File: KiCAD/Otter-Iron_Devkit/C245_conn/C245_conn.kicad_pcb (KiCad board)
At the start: 2 copper layers, 24.7 x 20.4 mm, 3 parts, among them J1 Otter-Iron, J2 C245

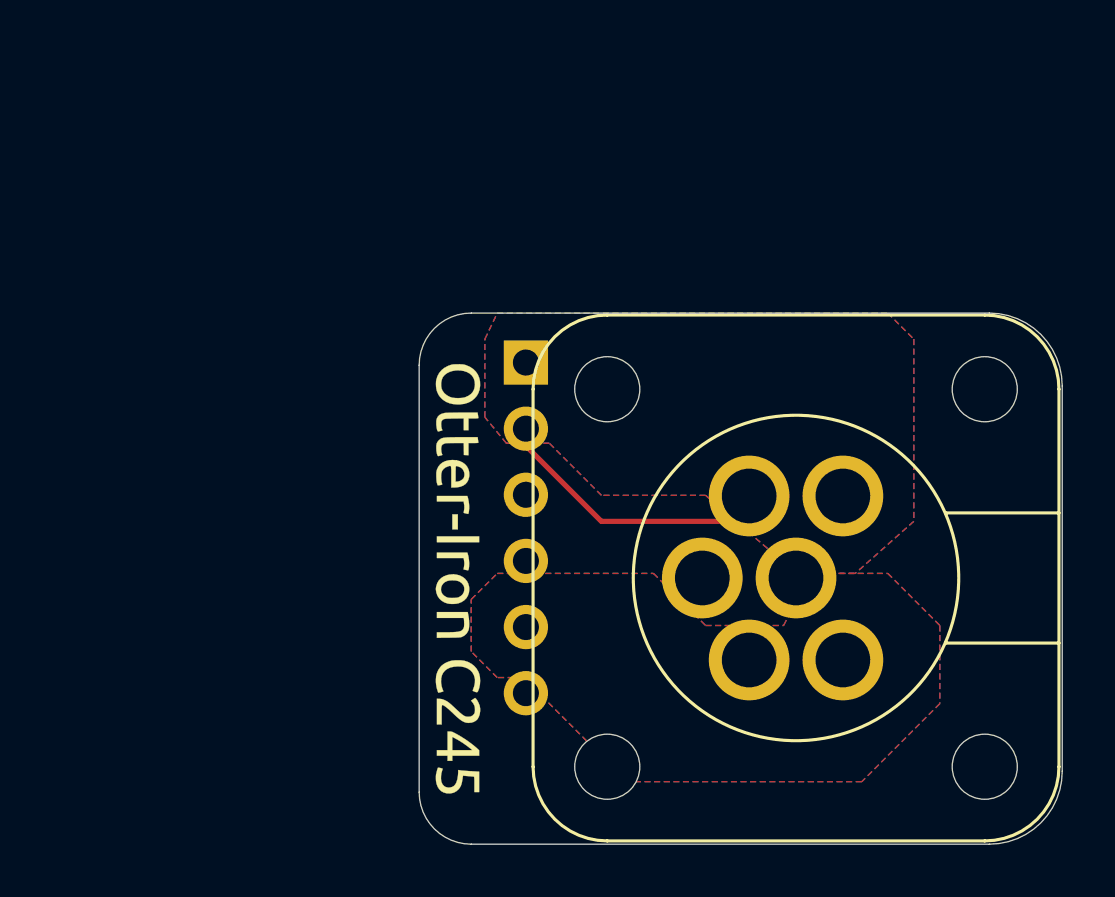
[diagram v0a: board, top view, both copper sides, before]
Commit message: added v2.0
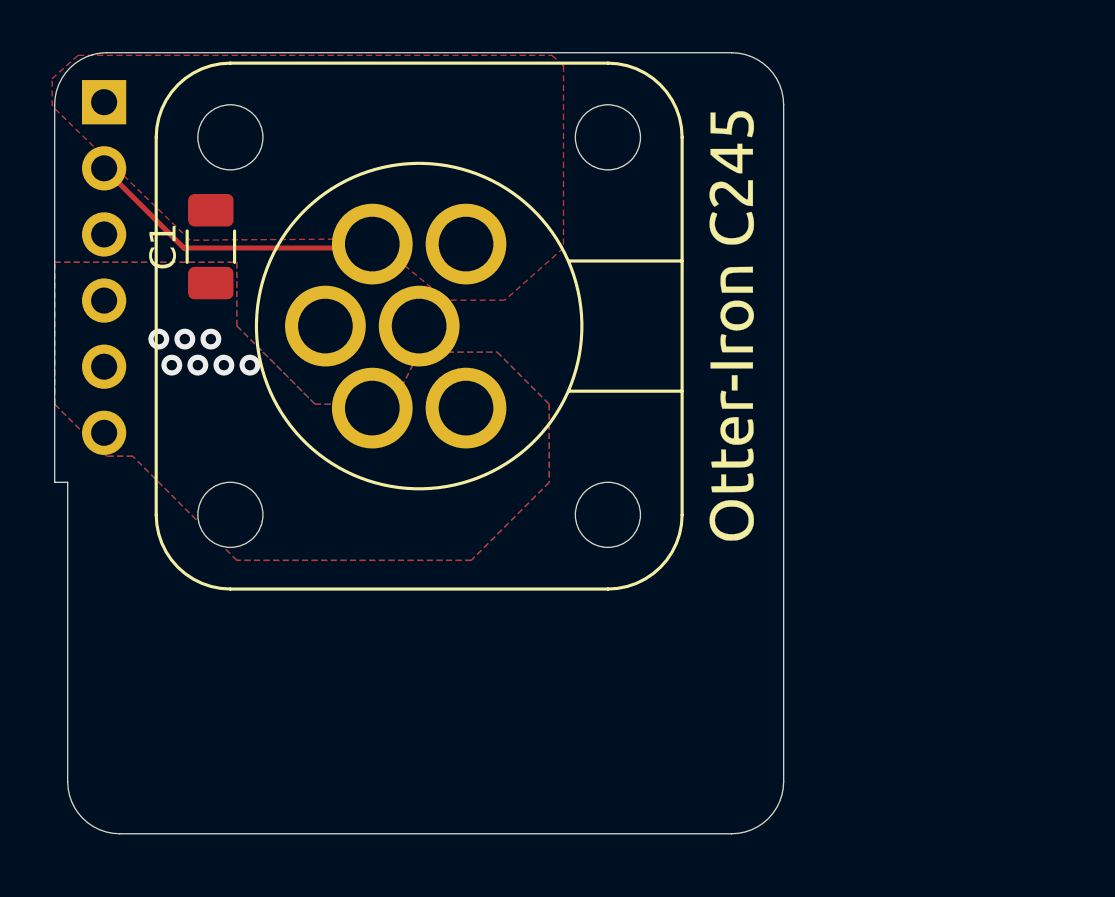
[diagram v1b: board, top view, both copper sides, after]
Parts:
- added C1: 10u, Capacitor_SMD:C_1206_3216Metric, F.Cu at (92.0, 97.5)
- J1: footprint Connector_PinHeader_2.54mm:PinHeader_1x06_P2.54mm_Horizontal -> Connector_PinHeader_2.54mm:PinHeader_1x06_P2.54mm_Vertical
- moved J1 19.0 mm to (87.9, 91.9)
- moved J2 17.4 mm to (100.0, 100.5)
- moved G*** 14.3 mm to (112.0, 100.5), turned to 90 degrees
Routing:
- net JUNC: track 10.9 -> 11.6 mm
- net HEAT: vias 0 -> 7
- removed copper zone on B.Cu, net GND
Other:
- board size 24.7 x 20.4 mm -> 28 x 30 mm
